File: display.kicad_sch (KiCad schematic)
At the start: 26 parts, among them J3 FH34SRJ-24S-0.5SH_99_, Q1 ZXM61N03F, Q2 ZXM61N03F, SW1 Button-THT - 2-1825910-7, U2 NCP1117LPST33T3G

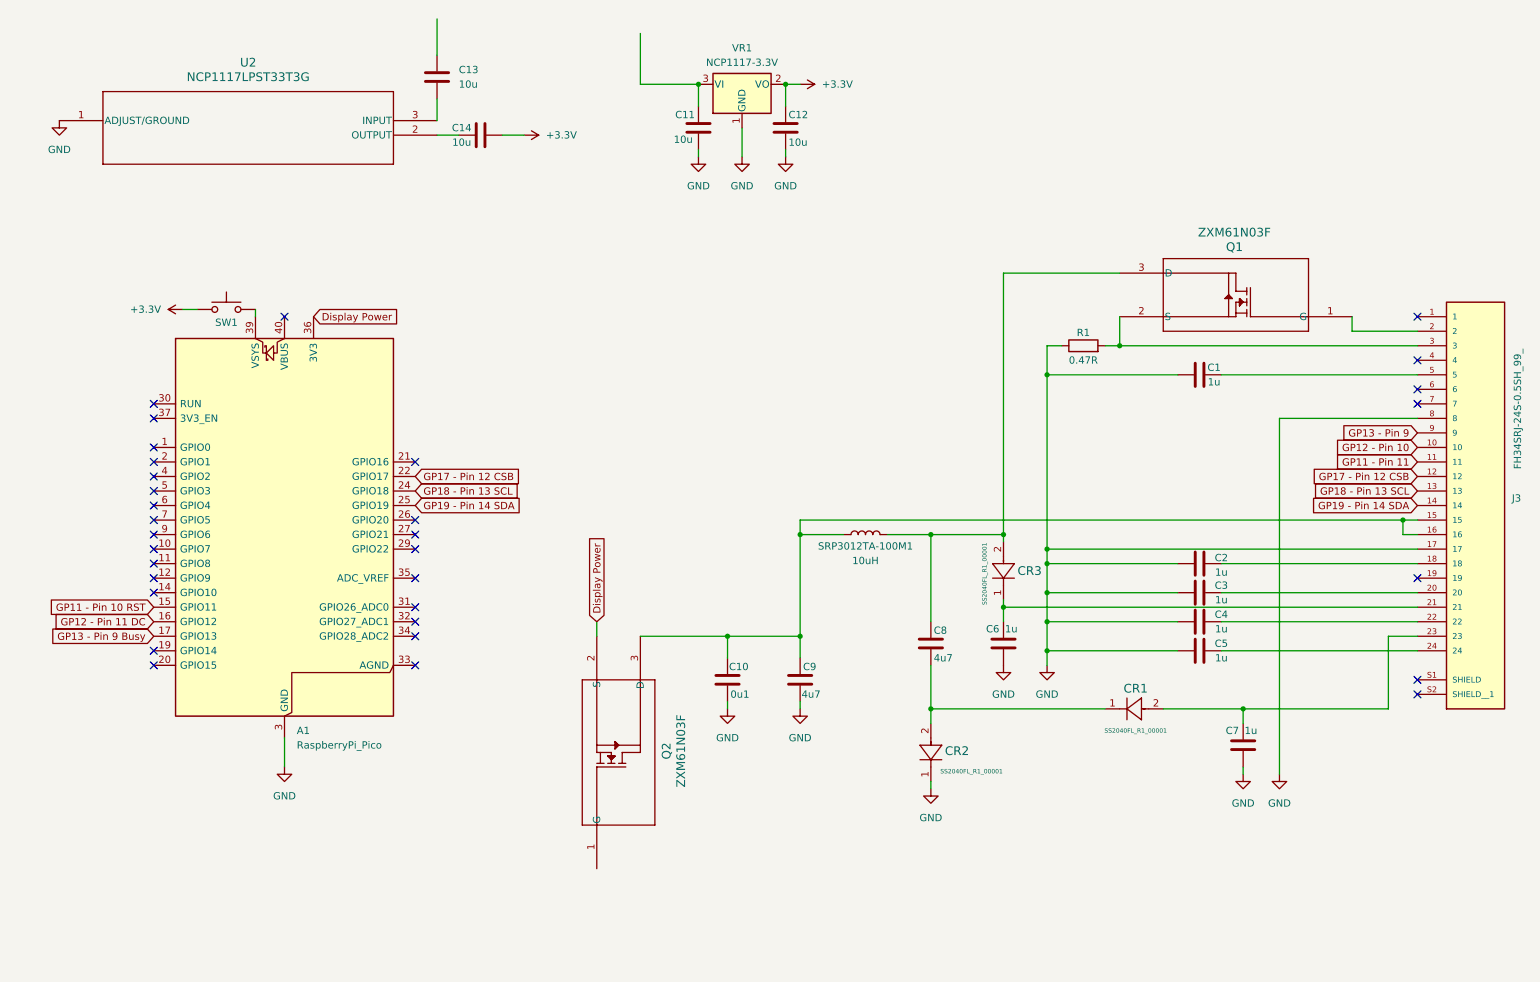
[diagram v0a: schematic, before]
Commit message: new
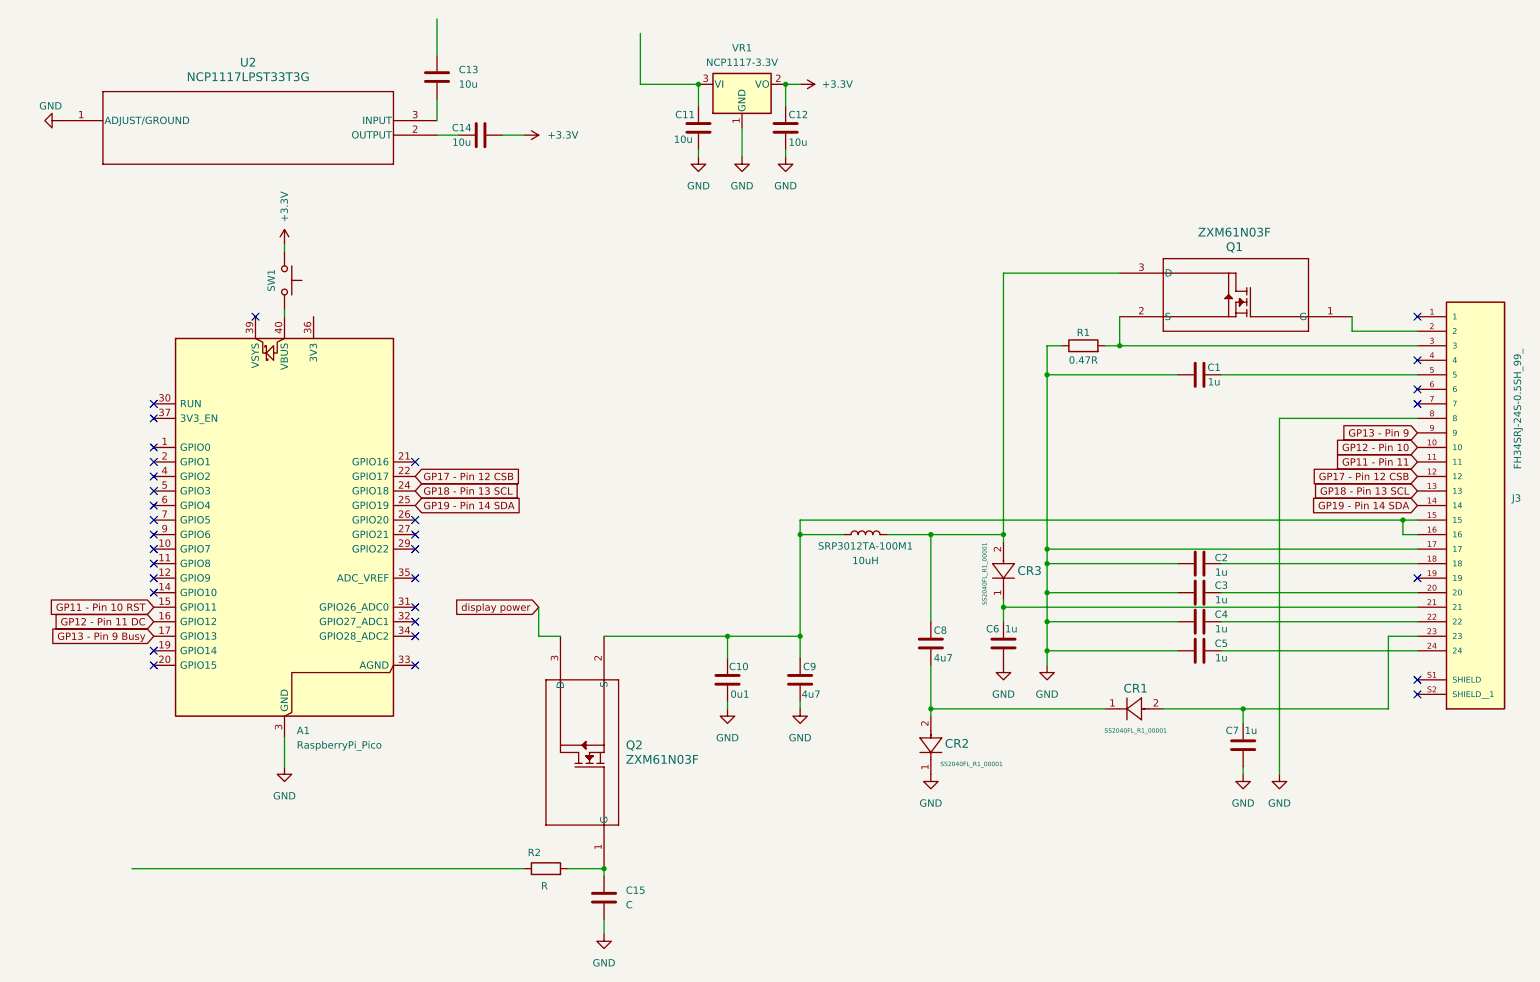
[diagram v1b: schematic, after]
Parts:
- added C15: C, symbol Device:C
- added R2: R, symbol Device:R
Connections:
- net GND: now also C15.2
- net at SW1.2: now also A1.40 (VBUS); no longer A1.39 (VSYS)
- net at C10.1, C9.1, J3.15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: now also Q2.2 (S); no longer Q2.3 (D)
- net at Q2.1 (G): now also C15.1, R2.2
- net Display Power: no longer names the net of A1.36 (3V3)
- net Display Power: no longer Q2.2 (S)
- new net display power: Q2.3 (D)
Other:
- moved on the sheet: CR2, SW1

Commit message: Update display.kicad_sch
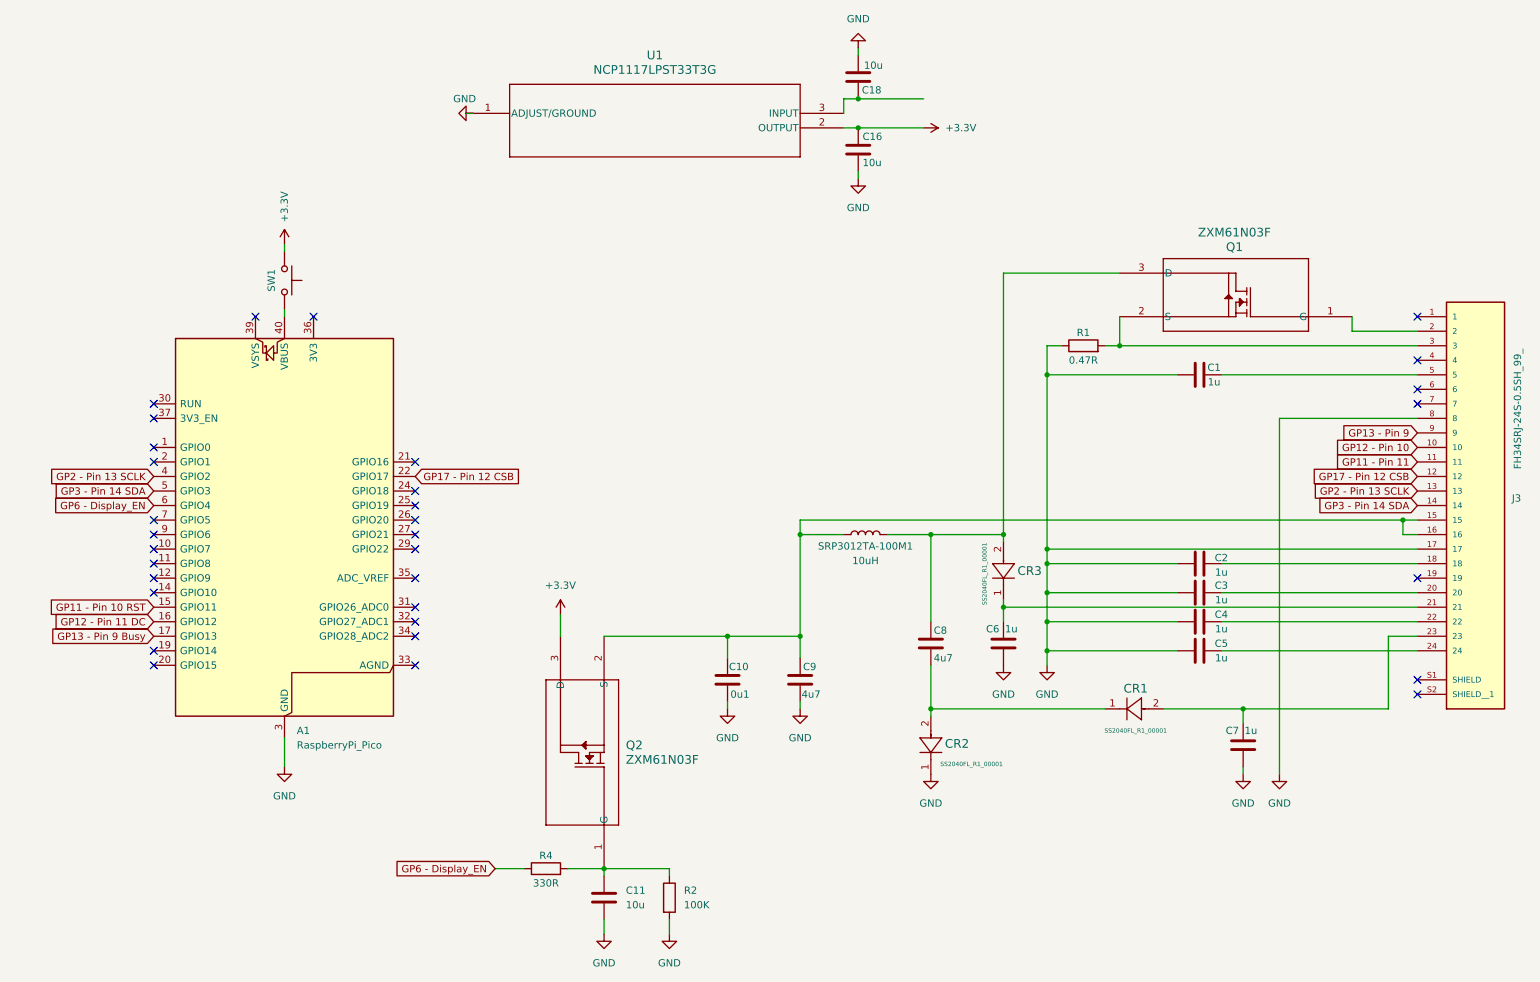
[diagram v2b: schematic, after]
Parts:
- removed C12, C13, C14: 10u, rsx_capacitors:C_0805_2012Metric, symbol rsx_Capacitors:10u
- removed C15: C, symbol Device:C
- removed R2: R, symbol Device:R
- removed U2: NCP1117LPST33T3G, SOT223-3_ONS, symbol NCP1117:NCP1117LPST33T3G
- removed VR1: NCP1117-3.3V, rsx_packages_TO_SOT:SOT-223-3_TabPin2, symbol rsx_voltage_regulation:NCP1117-3.3V
- added C16, C18: 10u, rsx_capacitors:C_0805_2012Metric, symbol rsx_Capacitors:10u
- added R2: 100K, rsx_resistors:R_0603_1608Metric, symbol rsx_Resistors:100K
- added R4: 330R, rsx_resistors:R_0603_1608Metric, symbol rsx_Resistors:330R
- added U1: NCP1117LPST33T3G, SOT223-3_ONS, symbol NCP1117:NCP1117LPST33T3G
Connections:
- net display power is gone; now on net +3.3V: Q2.3 (D)
- net +3.3V: now also C16.1, U1.2 (OUTPUT)
- net GND: now also C16.2, C18.2, R2.2, U1.1 (ADJUST/GROUND)
- net at Q2.1 (G): now also C11.1, R2.1, R4.2
- net GP2 - Pin 13 SCLK: now reaches A1.4 (GPIO2)
- net GP2 - Pin 13 SCLK: now also J3.13
- net GP3 - Pin 14 SDA: now reaches A1.5 (GPIO3)
- net GP3 - Pin 14 SDA: now also J3.14
- net GP6 - Display_EN: now reaches A1.6 (GPIO4)
- net GP6 - Display_EN: now also R4.1
- net GP18 - Pin 13 SCL: no longer names the net of A1.24 (GPIO18)
- net GP18 - Pin 13 SCL: no longer J3.13
- net GP19 - Pin 14 SDA: no longer names the net of A1.25 (GPIO19)
- net GP19 - Pin 14 SDA: no longer J3.14
- new net: C18.1, U1.3 (INPUT)

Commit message: 11/08/25
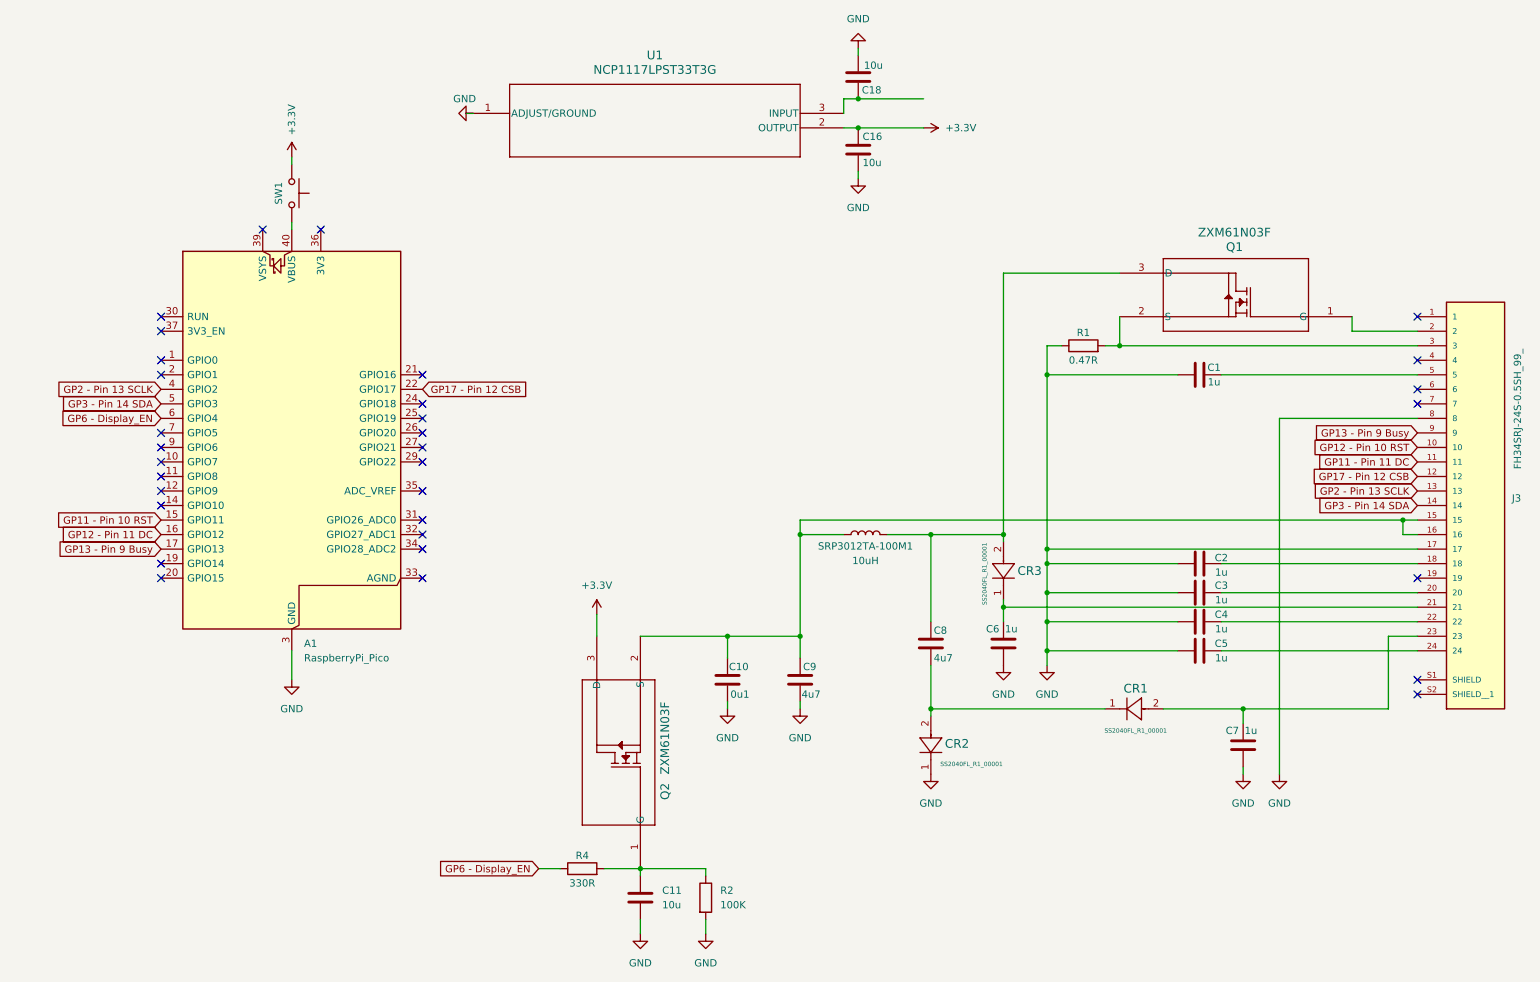
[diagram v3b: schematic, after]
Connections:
- net GP13 - Pin 9 is gone; now on net GP13 - Pin 9 Busy: J3.9
- net GP11 - Pin 11 renamed GP11 - Pin 11 DC
- net GP12 - Pin 10 renamed GP12 - Pin 10 RST
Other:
- moved on the sheet: A1, C11, Q2, R2, R4, SW1
